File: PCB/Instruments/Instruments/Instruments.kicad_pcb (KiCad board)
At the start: 2 copper layers, 38 x 55 mm, 8 parts, among them P1 Screw-Terminal-1x2, U1 SEEEDUINO XIAO, U2 LD33VT

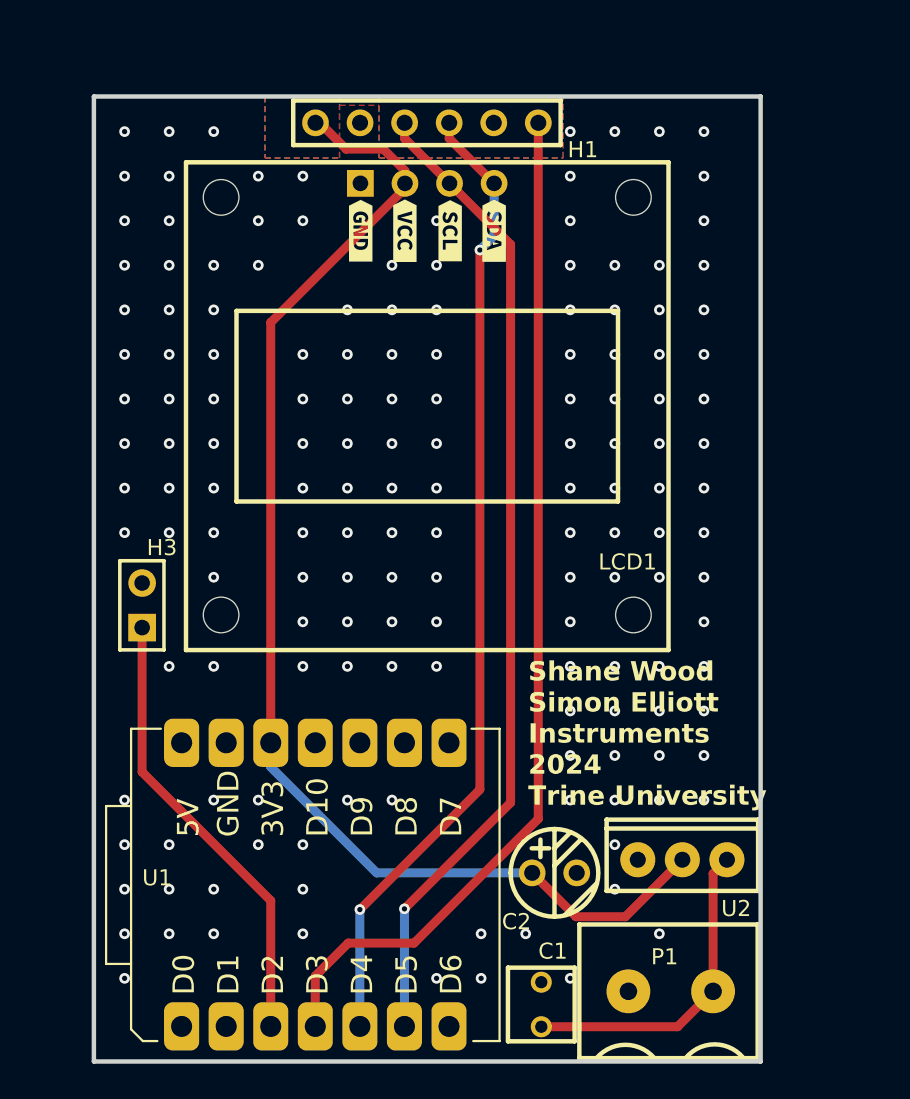
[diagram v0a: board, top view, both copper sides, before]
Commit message: Finished Code + PCB
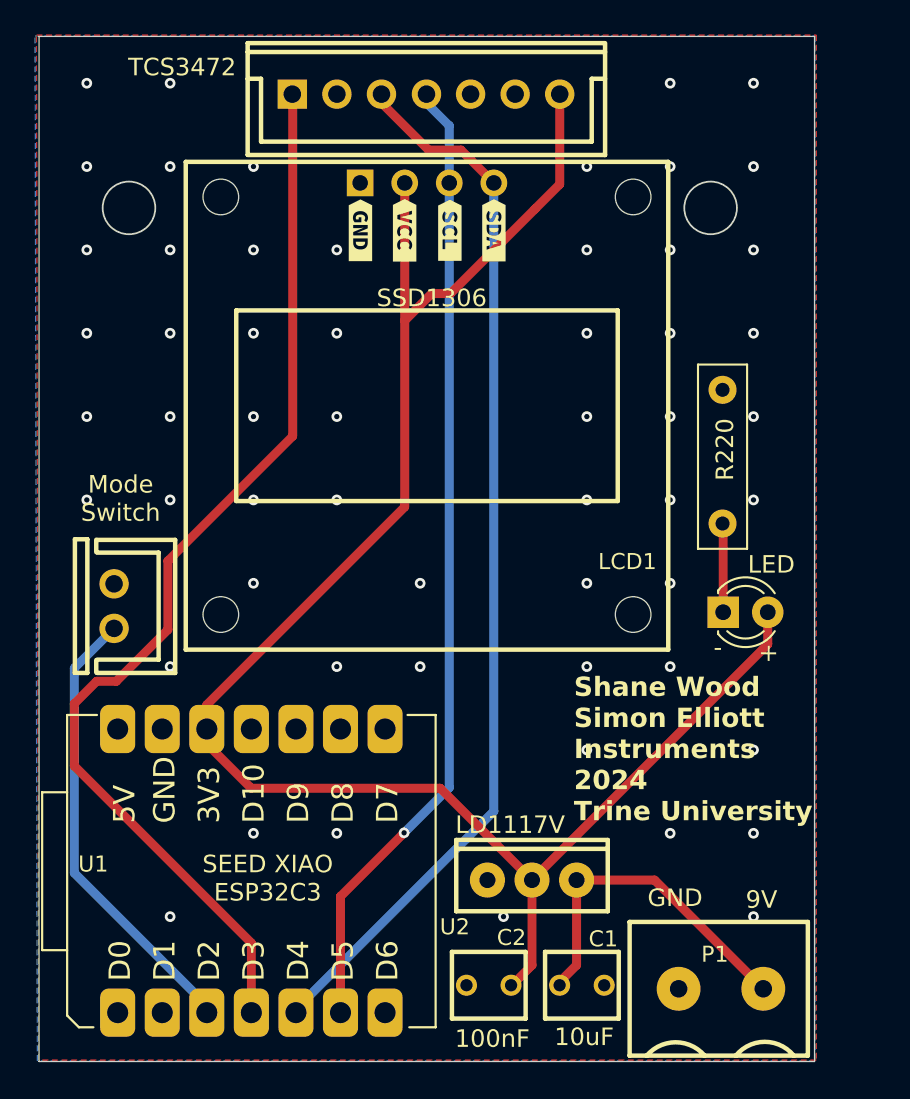
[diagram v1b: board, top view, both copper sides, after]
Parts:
- removed H1: 2.54mm 1*6P, Instruments:HDR-2.54-15-1X6P
- added D1: LED, LED_THT:LED_D3.0mm_IRBlack, F.Cu at (156.6, 96.4)
- added G***: LOGO, LOGO, B.Cu at (147.7, 84.1)
- added G***: LOGO, LOGO, B.Cu at (128.9, 83.1)
- added R1: R220, Resistor_THT:R_Array_SIP4, F.Cu at (156.6, 91.3)
- added U3: 7 pin JST Connector, Instruments:HDR-2.54-15-1X6P, F.Cu at (139.8, 70.5)
- C2: footprint Instruments:100UFX16V CAPACITOR D5.0XF11.0 -> Instruments:CAP-TH_L4.2-W3.8-P2.54-D0.5
- H3: value HDR-F-2.54_1x2 -> 2.54mm 1*2P
- LCD1: value SSD1306-OLED-128X64-I2C-VIZNY DEBORA -> SSD1306-OLED-128X64-I2C
- moved U2 8.65 mm to (143.2, 111.7)
- moved C2 7.42 mm to (143.3, 117.7)
- moved U1 3.73 mm to (140.2, 120.0)
- moved P1 2.87 mm to (153.2, 116.5)
- moved C1 2.56 mm to (148.6, 117.7), turned to 180 degrees
- moved H3 0.67 mm to (122.8, 96.1)
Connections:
- C2 pad 1: +3V3 -> GND
- C2 pad 2: GND -> +3V3
- U1 pad 1: (no net) -> unconnected-(U1-A0-Pad1)
- U1 pad 10: (no net) -> unconnected-(U1-D9-Pad10)
- U1 pad 11: (no net) -> unconnected-(U1-D10-Pad11)
- U1 pad 14: (no net) -> unconnected-(U1-5V-Pad14)
- U1 pad 2: (no net) -> unconnected-(U1-D1-Pad2)
- U1 pad 7: (no net) -> unconnected-(U1-TX-Pad7)
- U1 pad 8: (no net) -> unconnected-(U1-RX-Pad8)
- U1 pad 9: (no net) -> unconnected-(U1-D8-Pad9)
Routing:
- net +3V3: track 71.8 -> 102.9 mm
- net Net-(D1-K): track 0.00 -> 5.07 mm
- net SDA: track 56.0 -> 60.6 mm, vias 2 -> 0
- net LEDTCS: track 59.2 -> 61.8 mm
- net SCL: track 56.7 -> 54.9 mm
- net +9V: track 18.5 -> 19.4 mm
- net GND: vias 158 -> 56
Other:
- board size 38 x 55 mm -> 44.2 x 58.4 mm
- board text added: "+"
- board text added: "-"
- board text added: "100nF"
- board text added: "10uF"
- board text added: "3V3"
- board text added: "9V"
- board text added: "GND"
- board text added: "I2C Devices"
- board text added: "LD1117V"
- board text added: "LED X SDA SCL"
- board text added: "MicroController"
- board text added: "Mode Switch"
- board text added: "ModeSW"
- board text added: "Power Input"
- board text added: "SCL"
- board text added: "SDA"
- board text added: "SEED XIAO ESP32C3"
- board text added: "SSD1306"
- board text added: "TCS3472"
- board text added: "TCSLED"
- board text added: "User Input Switch"
- board text added: "X GND 3V3"
- board text removed: "3v3 Gnd SCL SDA x LED"
